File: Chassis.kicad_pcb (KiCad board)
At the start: 2 copper layers, 120 x 120 mm, 30 parts, among them IC1 RT6285GSP, J1 Conn_01x02, J10 Conn_01x02, J2 Conn_01x02, J3 Conn_01x02, J4 Conn_01x02, J5 Conn_01x02, J6 Conn_01x02, J7 Conn_01x02, J8 Conn_01x02, J9 Conn_01x02

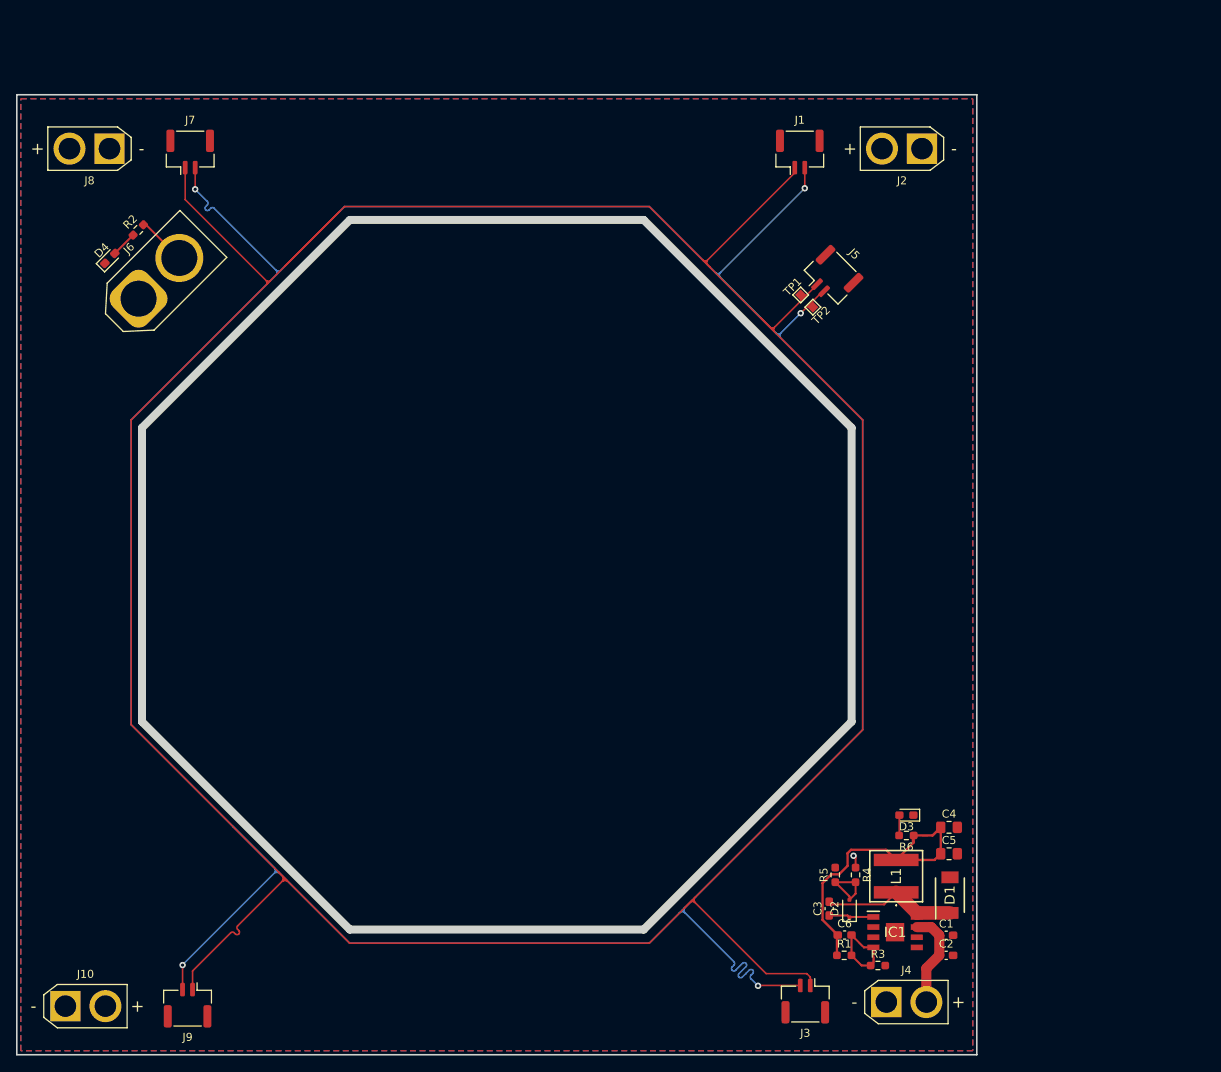
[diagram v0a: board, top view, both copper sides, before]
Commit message: Finalized board design
I think
Also added more 3D models and whatnot
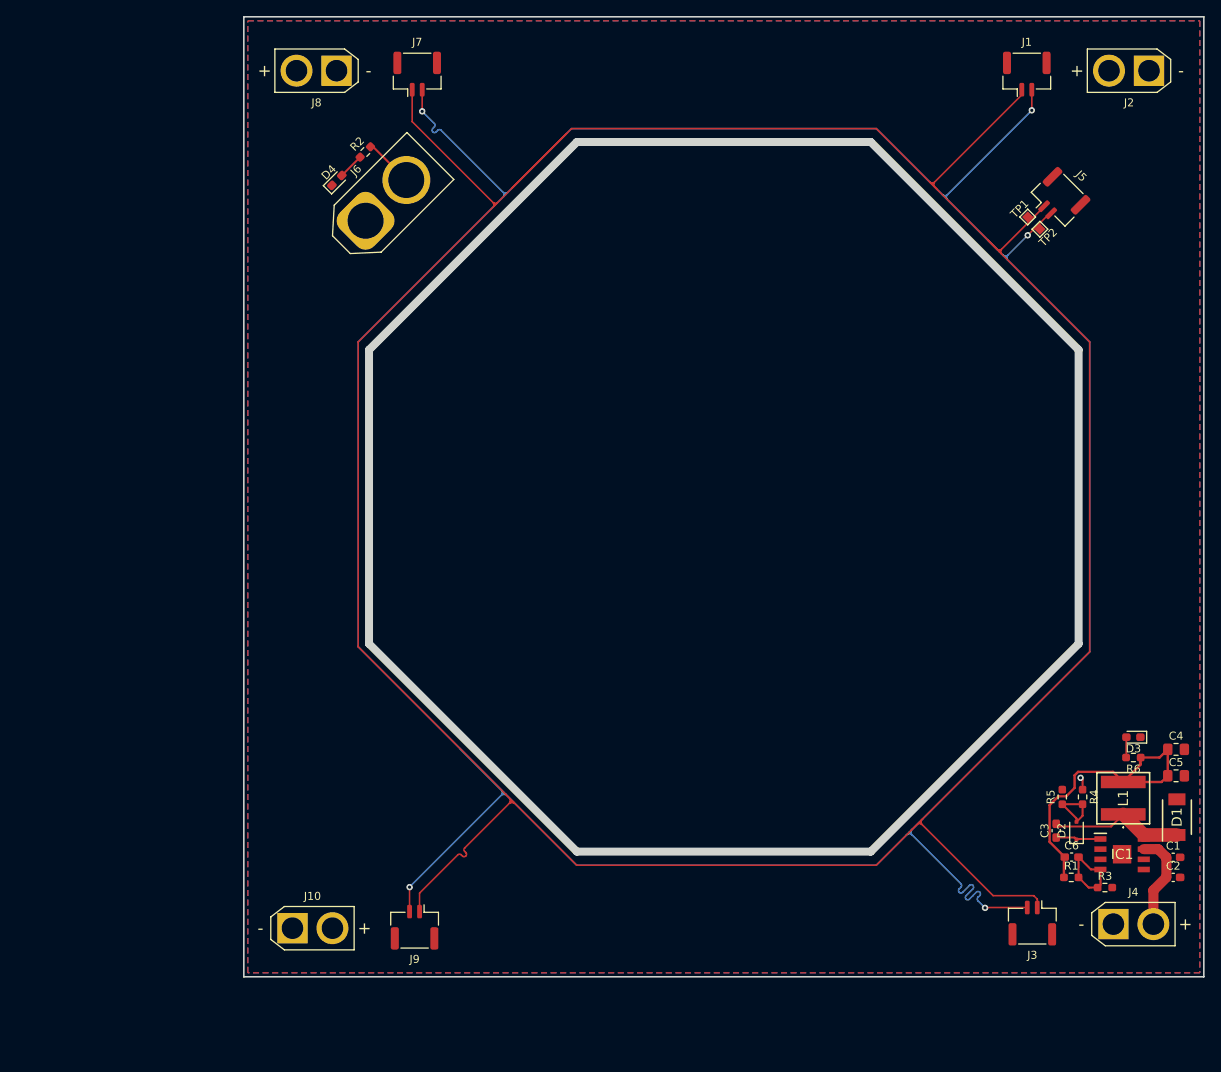
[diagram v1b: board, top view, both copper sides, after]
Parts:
- J10, J2, J4, J8: footprint Connector_AMASS:AMASS_XT30U-F_1x02_P5.0mm_Vertical -> Robomaster_ICs:AMASS_XT30U-F_1x02_P5.0mm_Vertical
- moved C1 30.0 mm to (204.6, 135.3)
- moved C2 30.0 mm to (204.6, 137.8)
- moved C4 30.0 mm to (204.9, 121.8)
- moved D1 30.0 mm to (205.0, 130.3)
- moved D2 30.0 mm to (192.5, 132.0)
- moved D3 30.0 mm to (199.6, 120.3)
- moved J10 30.0 mm to (94.5, 144.2)
- moved J4 30.0 mm to (197.1, 143.7)
- moved J9 30.0 mm to (109.7, 144.1)
- moved L1 30.0 mm to (198.3, 127.9)
- moved R1 30.0 mm to (191.8, 137.8)
- moved R3 30.0 mm to (196.0, 139.1)
- moved R4 30.0 mm to (193.2, 127.8)
- moved C5 30.0 mm to (204.9, 125.1)
- moved J2 30.0 mm to (201.5, 37.0)
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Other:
- outline, holes or cut-outs redrawn
